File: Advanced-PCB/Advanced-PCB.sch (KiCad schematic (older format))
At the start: 154 parts, among them J1 USB_mini_micro_B, SW1 Esc, SW10 Win 1.25, SW11 2, SW12 W, SW13 S, SW14 X, SW15 Alt 1.25, SW16 3, SW17 E, SW18 D, SW19 C, SW2 Tab 1.50, SW20 4, SW21 R, SW22 F, SW23 V, SW24 5, SW25 T, SW26 G, SW27 B, SW28 Space 6.25, SW29 6, SW3 Caps 1.75, SW30 Y, SW31 H, SW32 N, SW33 7, SW34 U, SW35 J, SW36 M, SW37 8, SW38 I, SW39 K, SW4 Shift 2.25, SW40 ,, SW41 9, SW42 P, SW43 L, SW44 ., SW45 Alt 1.25, SW46 0, SW47 O, SW48 ;, SW49 /, SW5 Ctrl 1.25, SW50 Fn 1.25, SW51 -, SW52 [, SW53 ', SW54 Shift 1.75, SW55 Left Arrow, SW56 =, SW57 ], SW58 Enter 2.25, SW59 Up Arrow, SW6 1, SW60 Down Arrow, SW61 Back 2.00, SW62 \\ 1.50, SW63 Pg Up, SW64 Pg Down, SW65 Right Arrow, SW66 `, SW67 Del, SW68 Alt 1.00, SW69 Fn 1.00, SW7 Q, SW70 Ctrl 1.00, SW8 A, SW9 Z, U1 ATMEGA32U4, X1 XTAL_GND

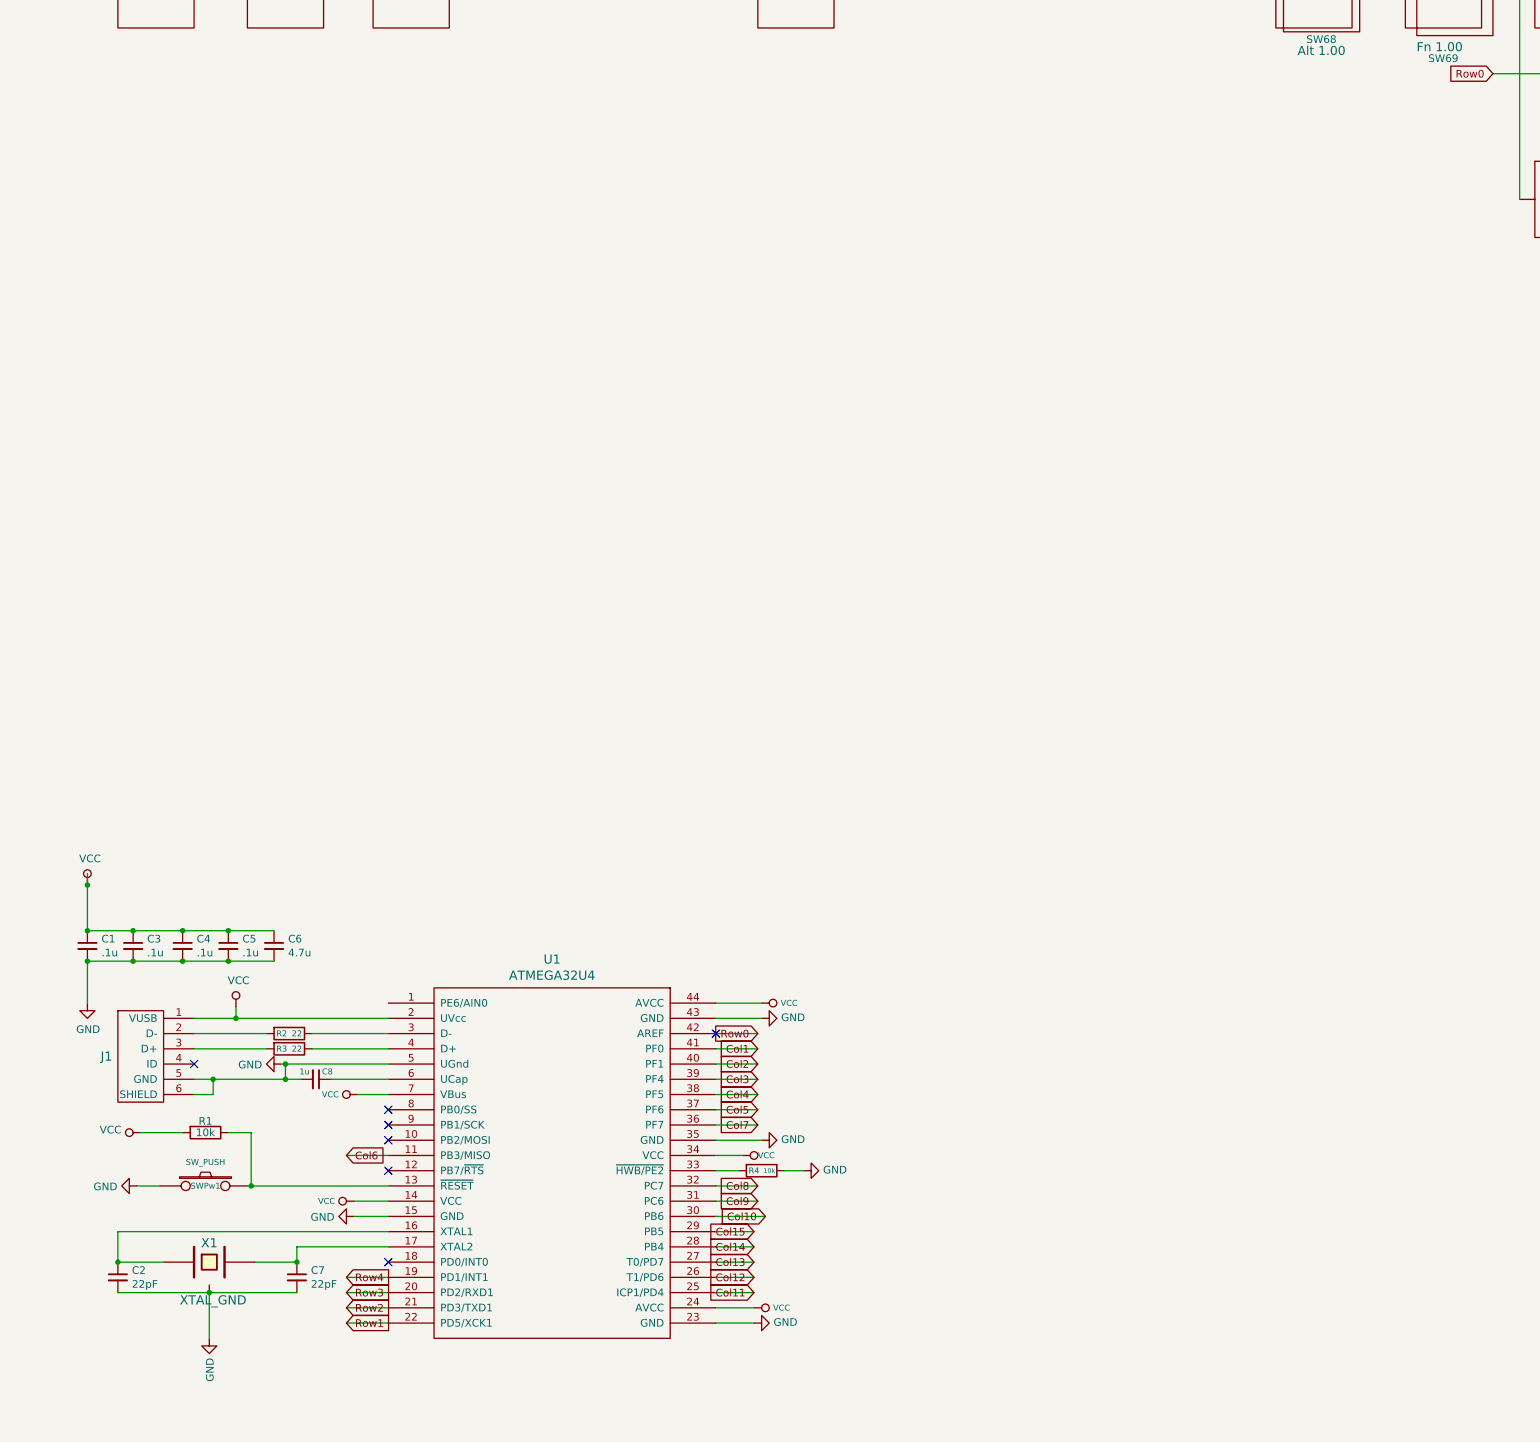
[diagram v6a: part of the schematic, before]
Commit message: BACKUP
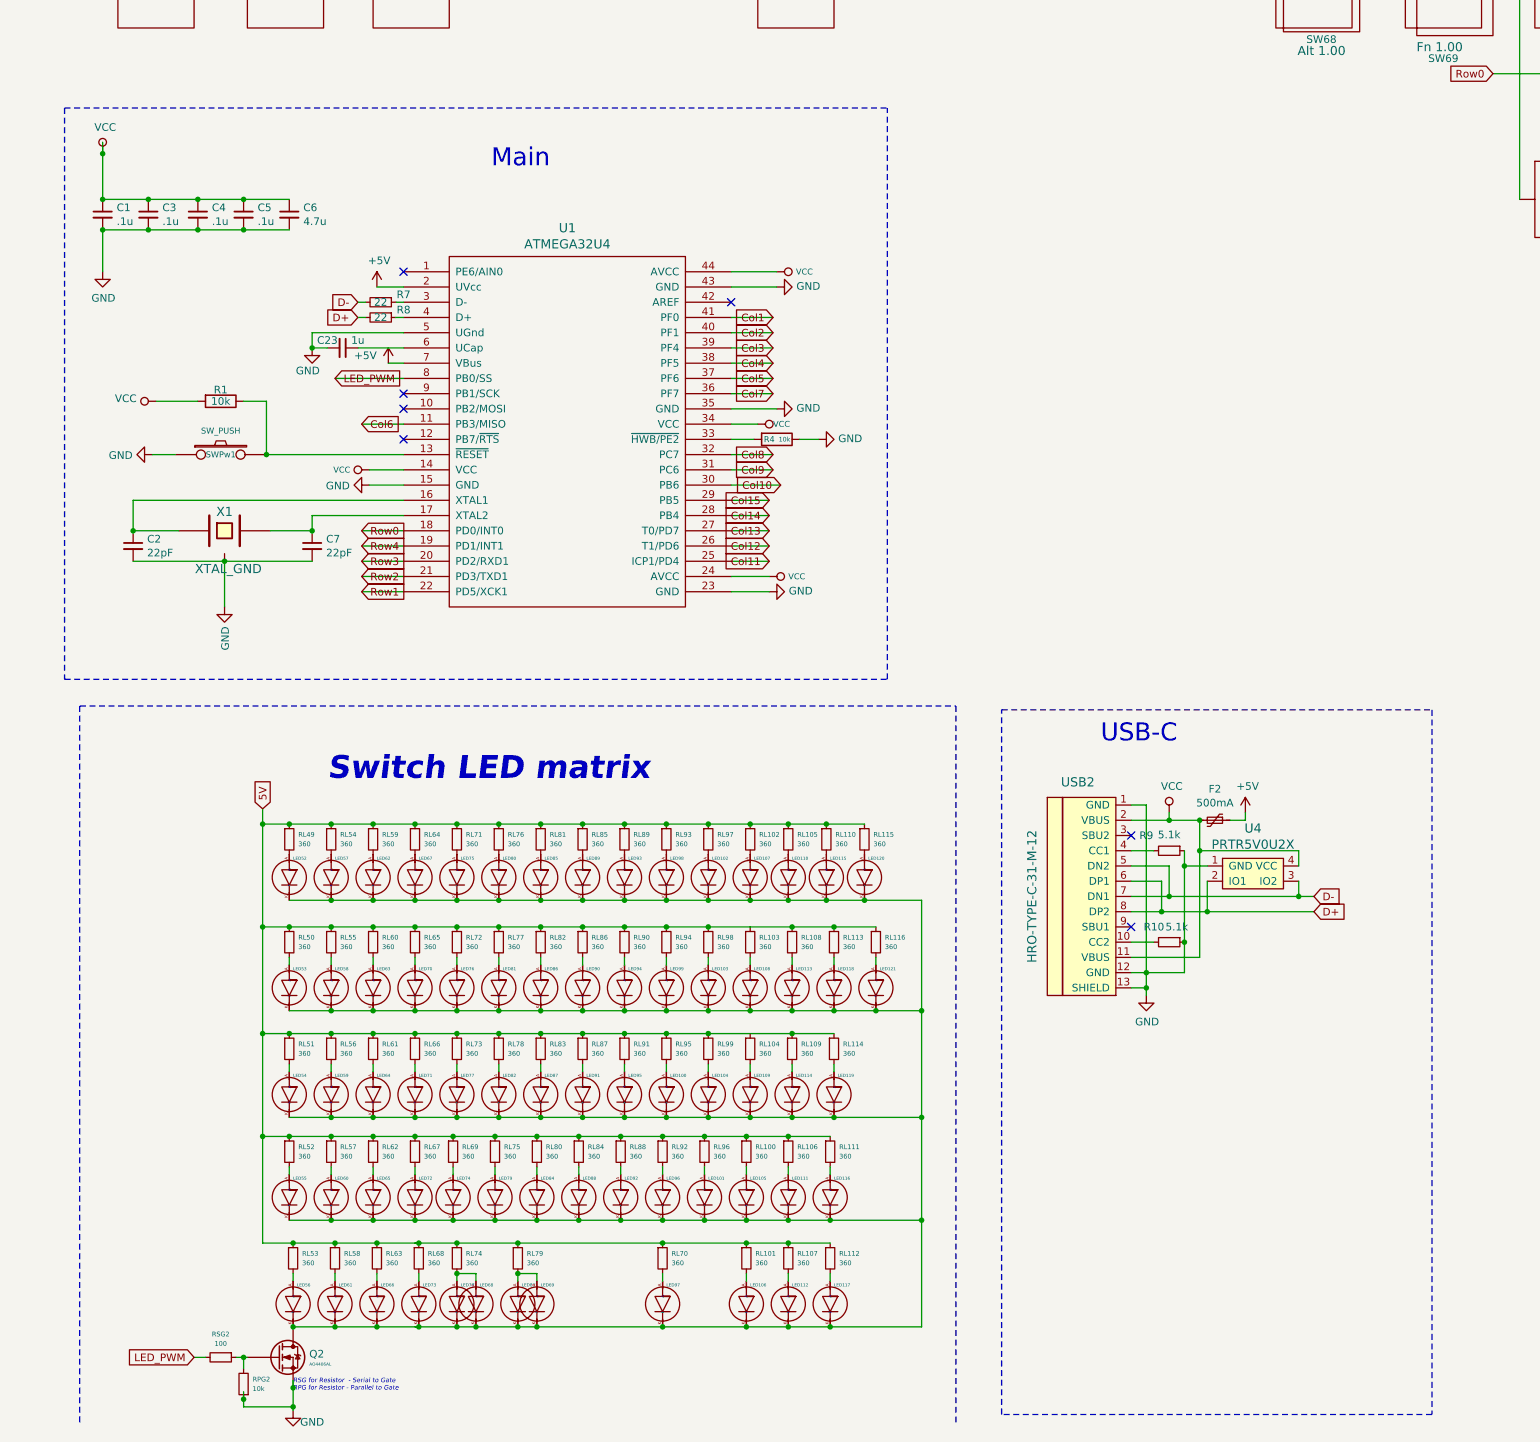
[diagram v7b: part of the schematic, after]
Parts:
- removed C8: 1u, Capacitor_SMD:C_0805_2012Metric_Pad1.15x1.40mm_HandSolder, symbol Device:C_Small
- removed J1: USB_mini_micro_B, acheron_Connectors:USB_MiniB_Hirose_UX60-MB-5S8, symbol Advanced-PCB-rescue:USB_mini_micro_B-keyboard_parts-Advanced-PCB-rescue
- removed R2, R3: 22, Resistor_SMD:R_0805_2012Metric_Pad1.15x1.40mm_HandSolder, symbol Device:R
- added C23: 1u, Capacitor_SMD:C_0603_1608Metric, symbol Device:C_Small
- added F2: 500mA, Resistor_SMD:R_0805_2012Metric, symbol Device:Polyfuse_Small
- added LED100, LED101, LED102, LED103, LED104, LED105, LED106, LED107, LED108, LED109, LED110, LED111, LED112, LED113, LED114, LED115, LED116, LED117, LED118, LED119, LED120, LED121, LED52, LED53, LED54, LED55, LED56, LED57, LED58, LED59, LED60, LED61, LED62, LED63, LED64, LED65, LED66, LED67, LED68, LED69, LED70, LED71, LED72, LED73, LED74, LED75, LED76, LED77, LED78, LED79, LED80, LED81, LED82, LED83, LED84, LED85, LED86, LED87, LED88, LED89, LED90, LED91, LED92, LED93, LED94, LED95, LED96, LED97, LED98, LED99: LED, LED_SMD:LED_WS2812B_PLCC4_5.0x5.0mm_P3.2mm, symbol acheronSymbols:LED
- added Q2: AO4406AL, acheronComponents:SOIC-8, symbol acheronSymbols:AO4406AL
- added R10, R9: 5.1k, Resistor_SMD:R_0603_1608Metric, symbol Device:R_Small
- added R7, R8: 22, Resistor_SMD:R_0603_1608Metric, symbol Device:R_Small
- added RL100, RL101, RL102, RL103, RL104, RL105, RL106, RL107, RL108, RL109, RL110, RL111, RL112, RL113, RL114, RL115, RL116, RL49, RL50, RL51, RL52, RL53, RL54, RL55, RL56, RL57, RL58, RL59, RL60, RL61, RL62, RL63, RL64, RL65, RL66, RL67, RL68, RL69, RL70, RL71, RL72, RL73, RL74, RL75, RL76, RL77, RL78, RL79, RL80, RL81, RL82, RL83, RL84, RL85, RL86, RL87, RL88, RL89, RL90, RL91, RL92, RL93, RL94, RL95, RL96, RL97, RL98, RL99: 360, acheronComponents:R_1026, symbol Device:R_Small
- added RPG2: 10k, acheronComponents:R_1026, symbol Device:R_Small
- added RSG2: 100, acheronComponents:R_1026, symbol Device:R_Small
- added U4: PRTR5V0U2X, random-keyboard-parts:SOT143B, symbol mullet-pcb-rescue:PRTR5V0U2X-ai03-locallib
- added USB2: HRO-TYPE-C-31-M-12, Type-C_Master:HRO-TYPE-C-31-M-12-HandSoldering, symbol mullet-pcb-rescue:HRO-TYPE-C-31-M-12-Type-C
- D1, D10, D11, D12, D13, D14, D15, D16, D17, D18, D19, D2, D20, D21, D22, D23, D24, D25, D26, D27, D28, D29, D3, D30, D31, D32, D33, D34, D35, D36, D37, D38, D39, D4, D40, D41, D42, D43, D44, D45, D46, D47, D48, D49, D5, D50, D51, D52, D53, D54, D55, D56, D57, D58, D59, D6, D60, D61, D62, D63, D64, D65, D66, D67, D7, D70, D8, D9: footprint Diode_SMD:D_SOD-123 -> keyboard-parts:D_SOD123_axial
- SW70: footprint acheron_MXA:MXA100 -> acheron_MX:MX100
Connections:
- net GND: now also C23.2, Q2.1, Q2.2, Q2.3, R10.1, R9.1, RPG2.1, U4.1 (GND), USB2.1 (GND), USB2.12 (GND), USB2.13 (SHIELD)
- net Row0: now also U1.18 (PD0/INT0); no longer U1.42 (AREF)
- net VCC: now also F2.2, U4.4 (VCC), USB2.11 (VBUS), USB2.2 (VBUS); no longer U1.2 (UVcc), U1.7 (VBus)
- net at U1.3 (D-): now also R7.1
- net at U1.4 (D+): now also R8.1
- net at U1.6 (UCap): now also C23.1
- net LED_PWM: now reaches U1.8 (PB0/SS)
- net LED_PWM: now also RSG2.2
- new net: LED110.A, RL105.2
- new net: LED100.K, LED101.K, LED102.K, LED103.K, LED104.K, LED105.K, LED106.K, LED107.K, LED108.K, LED109.K, LED110.K, LED111.K, LED112.K, LED113.K, LED114.K, LED115.K, LED116.K, LED117.K, LED118.K, LED119.K, LED120.K, LED121.K, LED52.K, LED53.K, LED54.K, LED55.K, LED56.K, LED57.K, LED58.K, LED59.K, LED60.K, LED61.K, LED62.K, LED63.K, LED64.K, LED65.K, LED66.K, LED67.K, LED68.K, LED69.K, LED70.K, LED71.K, LED72.K, LED73.K, LED74.K, LED75.K, LED76.K, LED77.K, LED78.K, LED79.K, LED80.K, LED81.K, LED82.K, LED83.K, LED84.K, LED85.K, LED86.K, LED87.K, LED88.K, LED89.K, LED90.K, LED91.K, LED92.K, LED93.K, LED94.K, LED95.K, LED96.K, LED97.K, LED98.K, LED99.K, Q2.5 (D), Q2.6, Q2.7, Q2.8
- new net: LED115.A, RL110.2
- new net: LED120.A, RL115.2
- new net: LED52.A, RL49.2
- new net: LED57.A, RL54.2
- new net: LED62.A, RL59.2
- new net: LED67.A, RL64.2
- new net: LED75.A, RL71.2
- new net: LED80.A, RL76.2
- new net: LED85.A, RL81.2
- new net: LED89.A, RL85.2
- new net: LED93.A, RL89.2
- new net: LED98.A, RL93.2
- new net: LED102.A, RL97.2
- new net: LED107.A, RL102.2
- new net: LED53.A, RL50.2
- new net: LED58.A, RL55.2
- new net: LED63.A, RL60.2
- new net: LED70.A, RL65.2
- new net: LED76.A, RL72.2
- new net: LED81.A, RL77.2
- new net: LED86.A, RL82.2
- new net: LED90.A, RL86.2
- new net: LED94.A, RL90.2
- new net: LED99.A, RL94.2
- new net: LED103.A, RL98.2
- new net: LED108.A, RL103.2
- new net: LED54.A, RL51.2
- new net: LED59.A, RL56.2
- new net: LED64.A, RL61.2
- new net: LED71.A, RL66.2
- new net: LED77.A, RL73.2
- new net: LED82.A, RL78.2
- new net: LED87.A, RL83.2
- new net: LED91.A, RL87.2
- new net: LED95.A, RL91.2
- new net: LED100.A, RL95.2
- new net: LED104.A, RL99.2
- new net: LED109.A, RL104.2
- new net: LED55.A, RL52.2
- new net: LED60.A, RL57.2
- new net: LED65.A, RL62.2
- new net: LED72.A, RL67.2
- new net: Q2.4 (G), RPG2.2, RSG2.1
- new net: LED113.A, RL108.2
- new net: LED118.A, RL113.2
- new net: LED121.A, RL116.2
- new net: LED114.A, RL109.2
- new net: LED119.A, RL114.2
- new net: LED74.A, RL69.2
- new net: LED79.A, RL75.2
- new net: LED84.A, RL80.2
- new net: LED88.A, RL84.2
- new net: LED92.A, RL88.2
- new net: LED96.A, RL92.2
- new net: LED101.A, RL96.2
- new net: LED105.A, RL100.2
- new net: LED111.A, RL106.2
- new net: LED116.A, RL111.2
- new net: LED56.A, RL53.2
- new net: LED61.A, RL58.2
- new net: LED66.A, RL63.2
- new net: LED73.A, RL68.2
- new net: LED106.A, RL101.2
- new net: LED112.A, RL107.2
- new net: LED117.A, RL112.2
- new net: LED68.A, LED78.A, RL74.2
- new net: LED69.A, LED83.A, RL79.2
- new net: LED97.A, RL70.2
- new net: R10.2, USB2.10 (CC2)
- new net: R9.2, USB2.4 (CC1)
- new net +5V: F2.1, U1.2 (UVcc), U1.7 (VBus)
- new net 5V: RL100.1, RL101.1, RL102.1, RL103.1, RL104.1, RL105.1, RL106.1, RL107.1, RL108.1, RL109.1, RL110.1, RL111.1, RL112.1, RL113.1, RL114.1, RL115.1, RL116.1, RL49.1, RL50.1, RL51.1, RL52.1, RL53.1, RL54.1, RL55.1, RL56.1, RL57.1, RL58.1, RL59.1, RL60.1, RL61.1, RL62.1, RL63.1, RL64.1, RL65.1, RL66.1, RL67.1, RL68.1, RL69.1, RL70.1, RL71.1, RL72.1, RL73.1, RL74.1, RL75.1, RL76.1, RL77.1, RL78.1, RL79.1, RL80.1, RL81.1, RL82.1, RL83.1, RL84.1, RL85.1, RL86.1, RL87.1, RL88.1, RL89.1, RL90.1, RL91.1, RL92.1, RL93.1, RL94.1, RL95.1, RL96.1, RL97.1, RL98.1, RL99.1
- new net D+: R8.2, U4.2 (IO1), USB2.6 (DP1), USB2.8 (DP2)
- new net D-: R7.2, U4.3 (IO2), USB2.5 (DN2), USB2.7 (DN1)
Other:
- note added: "Main\n"
- note added: "RSG for Resistor - Serial to Gate\nRPG for Resistor - Parallel to Gate"
- note added: "Switch LED matrix"
- note added: "USB-C"
- moved on the sheet: C1, C2, C3, C4, C5, C6, C7, R1, R4, SWPw1, U1, X1
